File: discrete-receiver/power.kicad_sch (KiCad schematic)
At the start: 32 parts, among them J2 Optional 5V DC Jack, U11 Ag9905LP, U12 TPS7A20xxxDBV, U13 LM66100DCK, U14 LM66100DCK, U15 LM66100DCK, U8 AMS1117

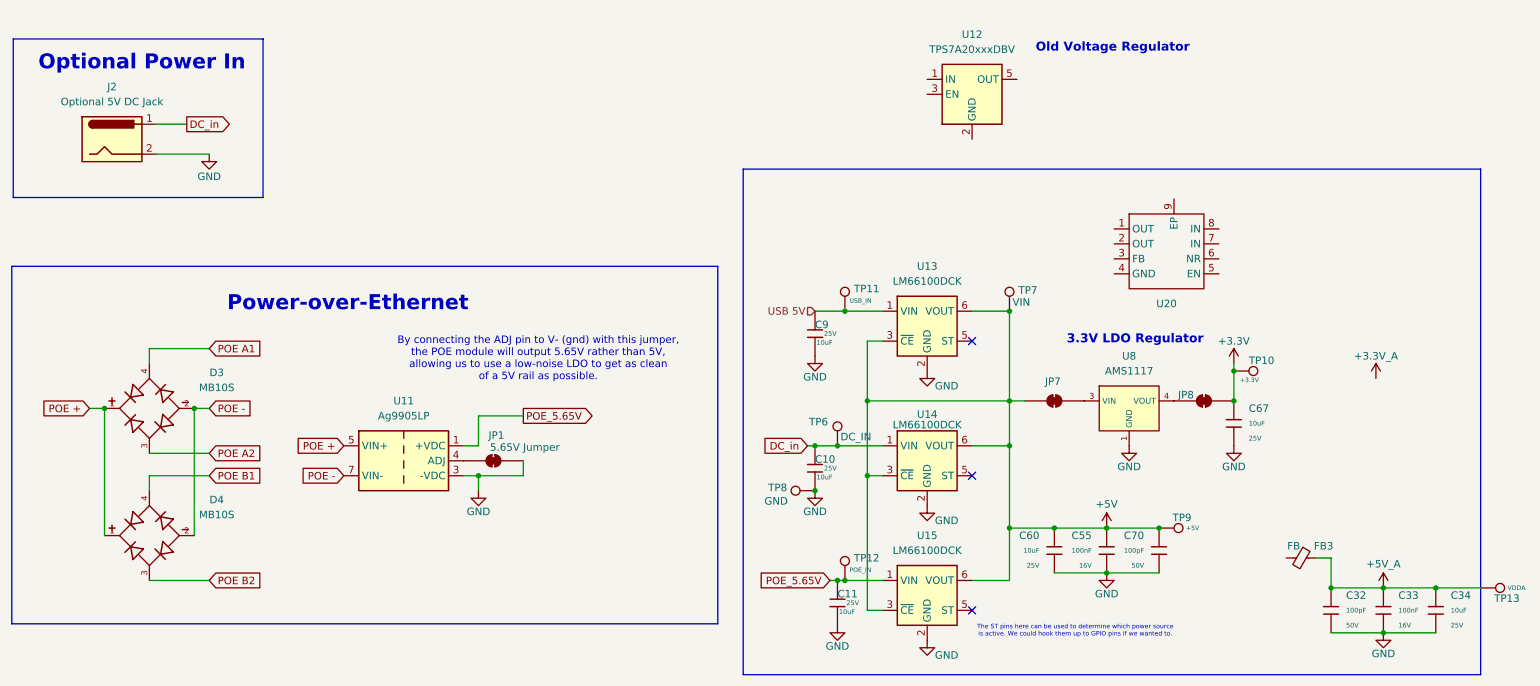
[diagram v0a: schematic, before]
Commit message: Progress on power design
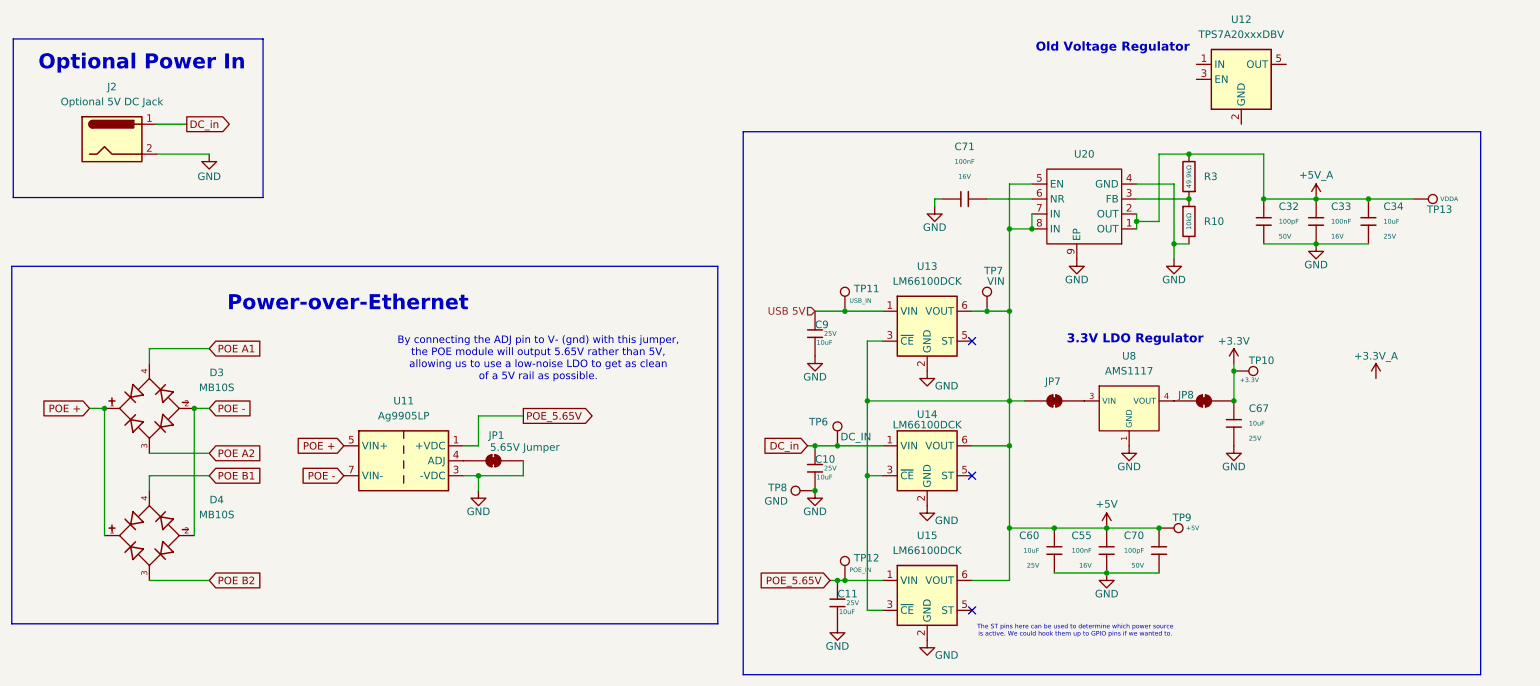
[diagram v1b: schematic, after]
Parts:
- removed FB3: FB, symbol Device:FerriteBead_Small
- added C71: 100nF, PCM_JLCPCB:C_0402, symbol PCM_JLCPCB-Capacitors:0402,100nF
- added R10: 10kΩ, PCM_JLCPCB:R_0402, symbol PCM_JLCPCB-Resistors:0402,10kΩ
- added R3: 49.9kΩ, PCM_JLCPCB:R_0402, symbol PCM_JLCPCB-Resistors:0402,49.9kΩ
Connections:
- net +5V: now also U20.5 (EN), U20.7 (IN), U20.8 (IN)
- net +5V_A: now also U20.1 (OUT), U20.2 (OUT), R3.2
- net GND: now also U20.4 (GND), U20.9 (EP), C71.1, R10.2
- net at U20.3 (FB): now also R10.1, R3.1
- net at U20.6 (NR): now also C71.2
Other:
- moved on the sheet: C32, C33, C34, TP13, TP7, U12, U20
